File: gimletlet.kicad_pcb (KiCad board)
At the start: 4 copper layers, 58 x 57 mm, 59 parts, among them J1 Conn_02x16_Odd_Even, J2 Conn_02x15_Odd_Even, J3 Conn_01x04, J4 SWD, J5 I2C, SW1 RESET, U1 STM32H753IITx, Y1 8MHz

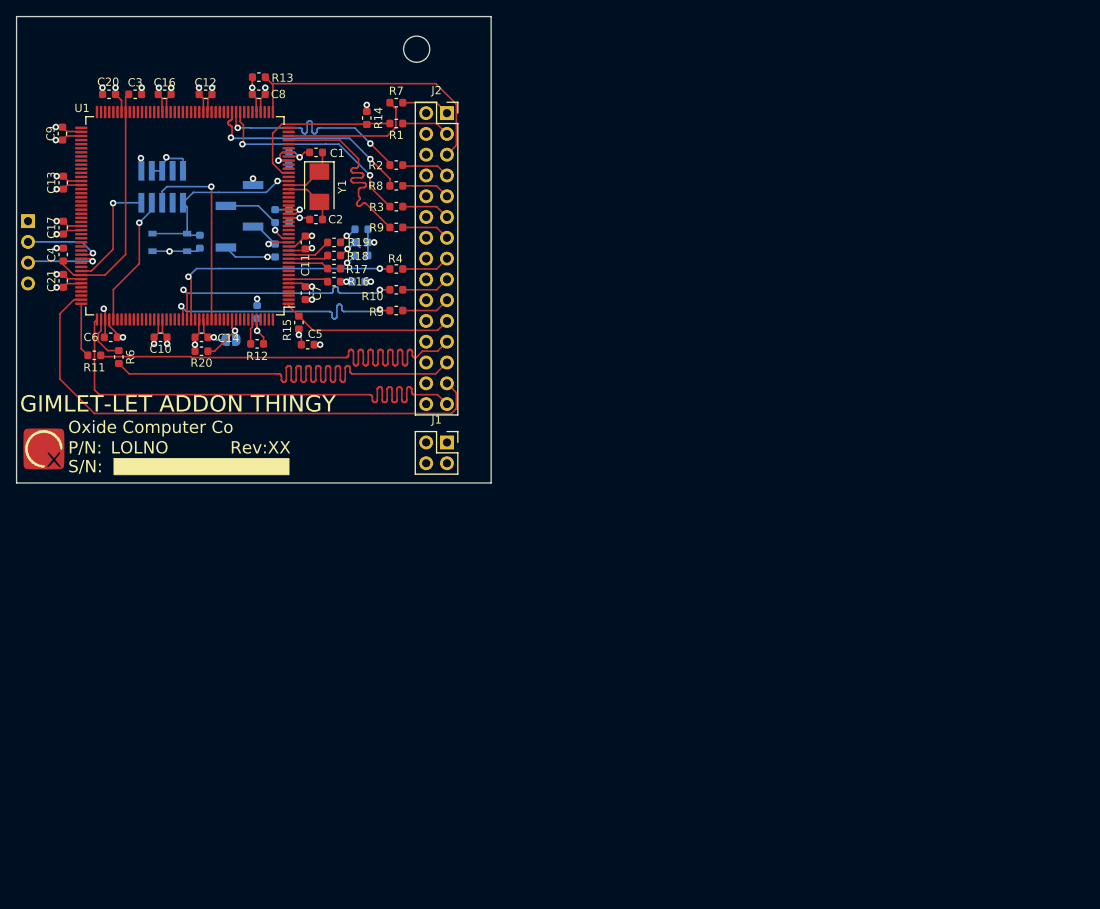
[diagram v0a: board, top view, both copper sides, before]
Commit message: gimletlet: revamp into useful board
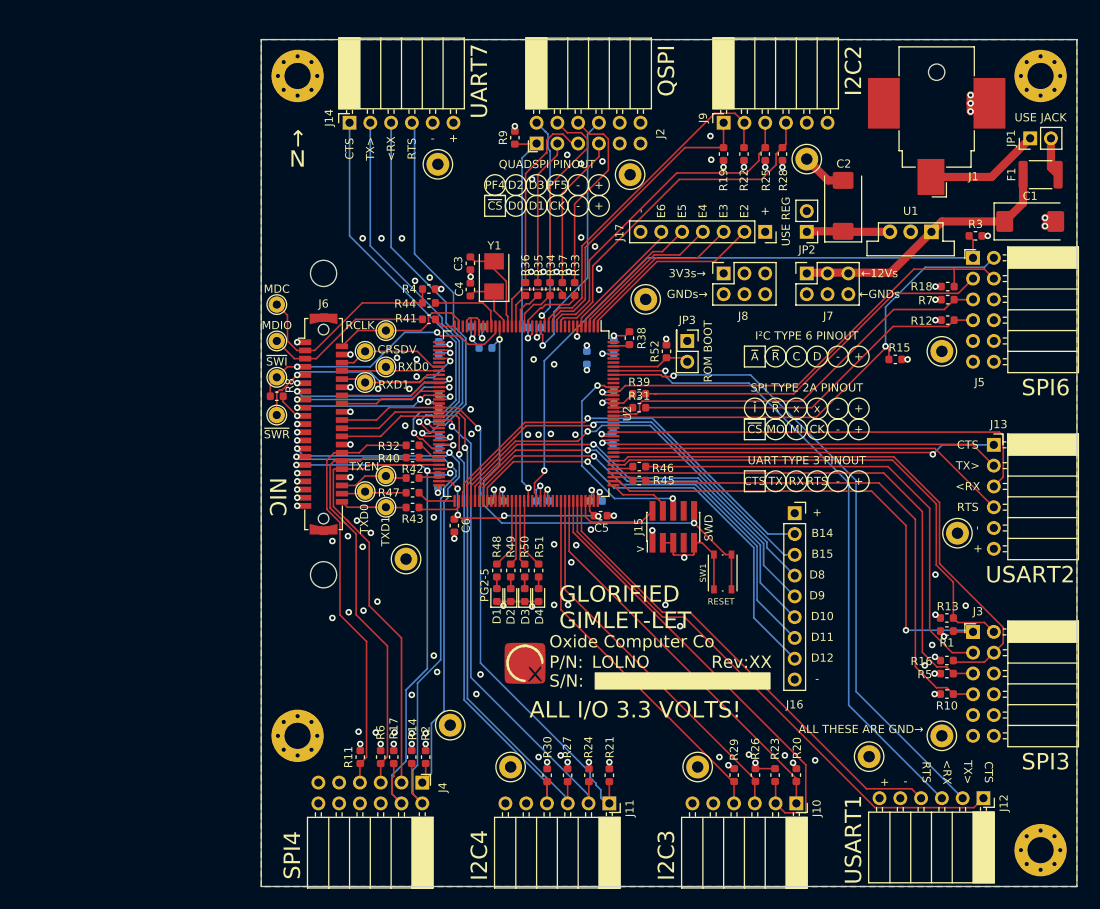
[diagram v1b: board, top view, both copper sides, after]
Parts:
- removed C21, C22: 0µ1, Capacitor_SMD:C_0603_1608Metric
- added F1: Polyfuse, Fuse:Fuse_1812_4532Metric, F.Cu at (184.2, 60.3)
- added H2: MountingHole, MountingHole:MountingHole_3.2mm_M3_Pad_Via, F.Cu at (184.2, 48.3)
- added H3: MountingHole, MountingHole:MountingHole_3.2mm_M3_Pad_Via, F.Cu at (184.2, 142.9)
- added H4: MountingHole, MountingHole:MountingHole_3.2mm_M3_Pad_Via, F.Cu at (93.3, 128.9)
- added H5: MountingHole, MountingHole:MountingHole_3.2mm_M3, F.Cu at (96.5, 72.4)
- added H6: MountingHole, MountingHole:MountingHole_3.2mm_M3, F.Cu at (96.5, 109.2)
- added J10: I2C3, pmod:PMOD_6pin_host_horizontal, F.Cu at (154.3, 137.2)
- added J11: I2C4, pmod:PMOD_6pin_host_horizontal, F.Cu at (131.4, 137.2)
- added J12: USART1, pmod:PMOD_6pin_host_horizontal, F.Cu at (177.2, 136.5)
- added J13: USART2, pmod:PMOD_6pin_host_horizontal, F.Cu at (178.4, 93.3)
- added J14: UART7, pmod:PMOD_6pin_host_horizontal, F.Cu at (99.7, 54.0)
- added J15: SWD, Connector_PinHeader_1.27mm:PinHeader_2x05_P1.27mm_Vertical_SMD, F.Cu at (139.3, 103.4)
- added J16: GPIO1, Connector_PinSocket_2.54mm:PinSocket_1x09_P2.54mm_Vertical, F.Cu at (154.1, 101.7)
- added J17: Conn_01x07, Connector_PinSocket_2.54mm:PinSocket_1x07_P2.54mm_Vertical, F.Cu at (150.5, 67.3)
- added J6: NIC, hirose-df9:Hirose_DF9-41S-1V(69)_2Rows_41Pin-2MP_P1.0mm_Vertical, F.Cu at (96.5, 90.8)
- added J7: 12V, Connector_PinSocket_2.54mm:PinSocket_2x03_P2.54mm_Vertical, F.Cu at (155.6, 72.4)
- added J8: 3V3, Connector_PinSocket_2.54mm:PinSocket_2x03_P2.54mm_Vertical, F.Cu at (145.4, 72.4)
- added J9: I2C2, pmod:PMOD_6pin_host_horizontal, F.Cu at (145.4, 54.0)
- added JP2: REG, Connector_PinHeader_2.54mm:PinHeader_1x02_P2.54mm_Vertical, F.Cu at (155.6, 67.3)
- added JP3: ROM, Connector_PinHeader_2.54mm:PinHeader_2x01_P2.54mm_Vertical, F.Cu at (141.0, 80.6)
- added R10: 10k, Resistor_SMD:R_0603_1608Metric, F.Cu at (172.7, 123.8)
- added R23: 10k, Resistor_SMD:R_0603_1608Metric, F.Cu at (151.7, 133.7)
- added R24: 10k, Resistor_SMD:R_0603_1608Metric, F.Cu at (128.9, 133.7)
- added R25: 10k, Resistor_SMD:R_0603_1608Metric, F.Cu at (150.5, 57.8)
- added R26: 10k, Resistor_SMD:R_0603_1608Metric, F.Cu at (149.3, 133.7)
- added R27: 10k, Resistor_SMD:R_0603_1608Metric, F.Cu at (126.3, 133.7)
- added R28: 10k, Resistor_SMD:R_0603_1608Metric, F.Cu at (152.6, 57.8)
- added R29: 10k, Resistor_SMD:R_0603_1608Metric, F.Cu at (146.7, 133.7)
- added R30: 10k, Resistor_SMD:R_0603_1608Metric, F.Cu at (123.8, 133.7)
- added R31: 22, Resistor_SMD:R_0603_1608Metric, F.Cu at (135.1, 88.8)
- added R32: 22, Resistor_SMD:R_0603_1608Metric, F.Cu at (107.4, 93.4)
- added R33: 22, Resistor_SMD:R_0603_1608Metric, F.Cu at (127.2, 74.3)
- added R34: 22, Resistor_SMD:R_0603_1608Metric, F.Cu at (124.2, 74.3)
- added R35: 22, Resistor_SMD:R_0603_1608Metric, F.Cu at (122.7, 74.3)
- added R36: 22, Resistor_SMD:R_0603_1608Metric, F.Cu at (121.2, 74.3)
- added R37: 22, Resistor_SMD:R_0603_1608Metric, F.Cu at (125.7, 74.3)
- added R38: 10k, Resistor_SMD:R_0603_1608Metric, F.Cu at (133.9, 80.3)
- added R39: 22, Resistor_SMD:R_0603_1608Metric, F.Cu at (135.1, 87.1)
- added R40: 22, Resistor_SMD:R_0603_1608Metric, F.Cu at (107.4, 94.9)
- added R41: 22, Resistor_SMD:R_0603_1608Metric, F.Cu at (109.4, 78.0)
- added R42: 22, Resistor_SMD:R_0603_1608Metric, F.Cu at (107.4, 97.4)
- added R44: 22, Resistor_SMD:R_0603_1608Metric, F.Cu at (109.4, 76.0)
- added R45: 22, Resistor_SMD:R_0603_1608Metric, F.Cu at (135.1, 97.7)
- added R46: 22, Resistor_SMD:R_0603_1608Metric, F.Cu at (135.1, 96.0)
- added R47: 22, Resistor_SMD:R_0603_1608Metric, F.Cu at (107.4, 99.2)
- added R48: 68, Resistor_SMD:R_0603_1608Metric, F.Cu at (117.7, 108.7)
- added R49: 68, Resistor_SMD:R_0603_1608Metric, F.Cu at (119.4, 108.7)
- added R50: 68, Resistor_SMD:R_0603_1608Metric, F.Cu at (121.1, 108.7)
- added R51: 68, Resistor_SMD:R_0603_1608Metric, F.Cu at (122.8, 108.7)
- added R52: 10k, Resistor_SMD:R_0603_1608Metric, F.Cu at (138.4, 81.9)
- added TP1: TestPoint_Small, TestPoint:TestPoint_THTPad_D2.0mm_Drill1.0mm, F.Cu at (90.8, 76.2)
- added TP10: TestPoint_Small, TestPoint:TestPoint_THTPad_D2.0mm_Drill1.0mm, F.Cu at (104.1, 83.8)
- added TP11: TestPoint_Small, TestPoint:TestPoint_THTPad_D2.0mm_Drill1.0mm, F.Cu at (101.6, 85.7)
- added TP12: GND, TestPoint:TestPoint_Loop_D3.50mm_Drill1.4mm_Beaded, F.Cu at (110.5, 59.1)
- added TP13: GND, TestPoint:TestPoint_Loop_D3.50mm_Drill1.4mm_Beaded, F.Cu at (134.0, 60.3)
- added TP14: GND, TestPoint:TestPoint_Loop_D3.50mm_Drill1.4mm_Beaded, F.Cu at (155.6, 58.4)
- added TP15: GND, TestPoint:TestPoint_Loop_D3.50mm_Drill1.4mm_Beaded, F.Cu at (172.1, 81.9)
- added TP16: GND, TestPoint:TestPoint_Loop_D3.50mm_Drill1.4mm_Beaded, F.Cu at (174.0, 104.1)
- added TP17: GND, TestPoint:TestPoint_Loop_D3.50mm_Drill1.4mm_Beaded, F.Cu at (172.1, 128.9)
- added TP18: GND, TestPoint:TestPoint_Loop_D3.50mm_Drill1.4mm_Beaded, F.Cu at (163.2, 131.4)
- added TP19: GND, TestPoint:TestPoint_Loop_D3.50mm_Drill1.4mm_Beaded, F.Cu at (142.2, 132.7)
- added TP2: TestPoint_Small, TestPoint:TestPoint_THTPad_D2.0mm_Drill1.0mm, F.Cu at (90.8, 80.6)
- added TP20: GND, TestPoint:TestPoint_Loop_D3.50mm_Drill1.4mm_Beaded, F.Cu at (119.4, 132.7)
- added TP21: GND, TestPoint:TestPoint_Loop_D3.50mm_Drill1.4mm_Beaded, F.Cu at (112.0, 127.6)
- added TP22: GND, TestPoint:TestPoint_Loop_D3.50mm_Drill1.4mm_Beaded, F.Cu at (106.6, 107.3)
- added TP23: GND, TestPoint:TestPoint_Loop_D3.50mm_Drill1.4mm_Beaded, F.Cu at (135.9, 75.6)
- added TP3: TestPoint_Small, TestPoint:TestPoint_THTPad_D2.0mm_Drill1.0mm, F.Cu at (90.8, 85.1)
- added TP4: TestPoint_Small, TestPoint:TestPoint_THTPad_D2.0mm_Drill1.0mm, F.Cu at (90.8, 89.7)
- added TP5: TestPoint_Small, TestPoint:TestPoint_THTPad_D2.0mm_Drill1.0mm, F.Cu at (104.1, 97.2)
- added TP6: TestPoint_Small, TestPoint:TestPoint_THTPad_D2.0mm_Drill1.0mm, F.Cu at (101.6, 99.1)
- added TP7: TestPoint_Small, TestPoint:TestPoint_THTPad_D2.0mm_Drill1.0mm, F.Cu at (104.1, 101.0)
- added TP8: TestPoint_Small, TestPoint:TestPoint_THTPad_D2.0mm_Drill1.0mm, F.Cu at (104.1, 79.4)
- added TP9: TestPoint_Small, TestPoint:TestPoint_THTPad_D2.0mm_Drill1.0mm, F.Cu at (101.6, 81.9)
- added U1: OKI-78SR-3.3_1.5-W36-C, Converter_DCDC:Converter_DCDC_muRata_OKI-78SR_Vertical, F.Cu at (170.8, 67.3)
- C1, C2: value 11p -> 22µ; footprint Capacitor_SMD:C_0603_1608Metric -> Capacitor_Tantalum_SMD:CP_EIA-7343-31_Kemet-D
- C10, C11, C12, C13, C14, C16, C17, C20, C8, C9: moved to B.Cu
- C3, C4: value 2µ2 100mR -> 11p
- C5: value 4µ7 -> 2µ2 100mR
- C6: value 0µ1 -> 2µ2 100mR
- C7: value 0µ1 -> 4µ7; moved to B.Cu
- D1, D2, D3, D4, R21, R22, SW1: moved to F.Cu
- H1: footprint MountingHole:MountingHole_3.2mm_M3 -> MountingHole:MountingHole_3.2mm_M3_Pad_Via; moved to F.Cu
- J1: value Conn_02x16_Odd_Even -> 12V; footprint Connector_PinSocket_2.54mm:PinSocket_2x02_P2.54mm_Vertical -> Connector_BarrelJack:BarrelJack_CUI_PJ-036AH-SMT_Horizontal
- J2: value Conn_02x15_Odd_Even -> QSPI; footprint Connector_PinSocket_2.54mm:PinSocket_2x15_P2.54mm_Vertical -> pmod:PMOD_12pin_host_horizontal
- J3: value Conn_01x04 -> SPI3; footprint Connector_PinHeader_2.54mm:PinHeader_1x04_P2.54mm_Horizontal -> pmod:PMOD_12pin_host_horizontal; moved to F.Cu
- J4: value SWD -> SPI4; footprint Connector_PinHeader_1.27mm:PinHeader_2x05_P1.27mm_Vertical_SMD -> pmod:PMOD_12pin_host_horizontal; moved to F.Cu
- J5: value I2C -> SPI6; footprint Connector_PinHeader_2.54mm:PinHeader_1x04_P2.54mm_Vertical_SMD_Pin1Left -> pmod:PMOD_12pin_host_horizontal; moved to F.Cu
- JP1: value ROM -> JACK; footprint Jumper:SolderJumper-2_P1.3mm_Open_RoundedPad1.0x1.5mm -> Connector_PinHeader_2.54mm:PinHeader_1x02_P2.54mm_Vertical; moved to F.Cu
- R1, R11, R2, R3, R5, R6, R7, R9: value 22 -> 10k
- R13, R14, R15: value 100k -> 10k
- R16, R17, R18, R19: value 68 -> 10k
- R4, R8: value 22 -> 100k
- U2: renamed from U1; value STM32H753IITx -> STM32H753ZITx; footprint Package_QFP:LQFP-176_24x24mm_P0.5mm -> Package_QFP:LQFP-144_20x20mm_P0.5mm
- moved J3 125.9 mm to (175.9, 116.2), turned to 0 degrees
- moved R13 107.0 mm to (172.7, 114.5), turned to 180 degrees
- moved JP1 100.7 mm to (182.9, 55.9), turned to 90 degrees
- moved R1 91.5 mm to (172.7, 116.1), turned to 180 degrees
- moved J5 89.8 mm to (175.9, 70.5)
- moved R20 89.3 mm to (154.3, 133.7), turned to 90 degrees
- moved R16 88.1 mm to (172.7, 119.7)
- moved C1 87.7 mm to (182.9, 66.0), turned to 0 degrees
- moved R12 84.4 mm to (172.8, 78.1), turned to 180 degrees
- moved R5 80.6 mm to (172.7, 121.3), turned to 180 degrees
- moved J4 79.5 mm to (108.6, 134.6)
- moved SW1 78.8 mm to (145.3, 109.0), turned to 270 degrees
- moved R14 78.3 mm to (107.3, 131.5), turned to 90 degrees
- moved R21 76.0 mm to (131.4, 133.7), turned to 90 degrees
- moved R18 75.1 mm to (172.8, 74.0)
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- renumbered R10 to R43
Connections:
- C1 pad 1: /OSC_OUT -> +12V
- C2 pad 1: /OSC_IN -> /REG_3V3
- C20 pad 1: +3V3 -> /~RST
- C3 pad 1: Net-(C3-Pad1) -> /OSC_IN
- C4 pad 1: Net-(C3-Pad1) -> /OSC_OUT
- C5 pad 1: +3V3 -> Net-(C5-Pad1)
- C6 pad 1: +3V3 -> Net-(C5-Pad1)
- H1 pad 1: (no net) -> GND
- J1 pad 1: +3V3 -> /JACK_12V
- J1 pad 2: Net-(J1-Pad2) -> GND
- J1 pad 3: +3V3 -> Net-(J1-Pad3)
- J2 pad 1: /X_MDIO -> /~QSPI_CS
- J2 pad 10: GND -> /QSPI_XTRA10
- J2 pad 11: /X_RMII_CRS_DV -> GND
- J2 pad 12: GND -> +3V3
- J2 pad 2: GND -> /QSPI_IO0
- J2 pad 3: /X_MDC -> /QSPI_IO1
- J2 pad 4: GND -> /QSPI_CLK
- J2 pad 5: /~SMI_IRQ -> GND
- J2 pad 6: GND -> +3V3
- J2 pad 7: /X_RMII_RXD0 -> /QSPI_XTRA7
- J2 pad 8: GND -> /QSPI_IO2
- J2 pad 9: /X_RMII_RXD1 -> /QSPI_IO3
- J3 pad 1: +3V3 -> /~SPI3_CS
- J3 pad 2: /USART1_TX -> /SPI3_MOSI
- J3 pad 3: /USART1_RX -> /SPI3_MISO
- J3 pad 4: GND -> /SPI3_SCK
- J4 pad 1: +3V3 -> /~SPI4_CS
- J4 pad 10: /~RST -> Net-(J4-Pad10)
- J4 pad 2: /SWDIO -> /SPI4_MOSI
- J4 pad 3: GND -> /SPI4_MISO
- J4 pad 4: /SWCLK -> /SPI4_SCK
- J4 pad 6: /SWO -> +3V3
- J4 pad 7: Net-(J4-Pad7) -> /~SPI4_INT
- J4 pad 8: Net-(J4-Pad8) -> /~SPI4_RESET
- J4 pad 9: GND -> Net-(J4-Pad9)
- J5 pad 1: +3V3 -> /~SPI6_CS
- J5 pad 2: /SDA -> /SPI6_MOSI
- J5 pad 3: /SCL -> /SPI6_MISO
- J5 pad 4: GND -> /SPI6_SCK
- JP1 pad 1: +3V3 -> /JACK_12V
- JP1 pad 2: /BOOT0 -> /12V_IN
- R1 pad 1: /MDC -> /~SPI3_CS
- R1 pad 2: /X_MDC -> +3V3
- R11 pad 1: /SPI2_SCK -> /SPI4_SCK
- R11 pad 2: /X_SPI_SCK -> +3V3
- R12 pad 1: Net-(R12-Pad1) -> /SPI6_SCK
- R13 pad 1: +3V3 -> /~SPI3_INT
- R13 pad 2: /~SMI_IRQ -> +3V3
- R14 pad 1: +3V3 -> /~SPI4_INT
- R14 pad 2: /MDC -> +3V3
- R15 pad 1: +3V3 -> /~SPI6_INT
- R15 pad 2: /~SW_IRQ -> +3V3
- R16 pad 1: Net-(D1-Pad2) -> /~SPI3_RESET
- R16 pad 2: /LED0 -> +3V3
- R17 pad 1: Net-(D2-Pad2) -> /~SPI4_RESET
- R17 pad 2: /LED1 -> +3V3
- R18 pad 1: Net-(D3-Pad2) -> /~SPI6_RESET
- R18 pad 2: /LED2 -> +3V3
- R19 pad 1: Net-(D4-Pad2) -> /~I2C2_SMBA
- R19 pad 2: /LED3 -> +3V3
- R2 pad 1: /RMII_RXD0 -> /~SPI4_CS
- R2 pad 2: /X_RMII_RXD0 -> +3V3
- R20 pad 1: /BOOT0 -> /~I2C3_SMBA
- R20 pad 2: GND -> +3V3
- R21 pad 1: /SDA -> /~I2C4_SMBA
- R22 pad 1: /SCL -> /~I2C2_RESET
- R3 pad 1: /RMII_CRS_DV -> /~SPI6_CS
- R3 pad 2: /X_RMII_CRS_DV -> +3V3
- R4 pad 1: /RMII_TXD0 -> +3V3
- R4 pad 2: /X_RMII_TXD0 -> /MDC
- R43 pad 2: /X_RMII_TXD1 -> Net-(R43-Pad2)
- R5 pad 1: /RMII_TXEN -> /SPI3_MISO
- R5 pad 2: /X_RMII_TXEN -> +3V3
- R6 pad 1: /SPI2_MOSI -> /SPI4_MISO
- R6 pad 2: /X_SPI_MOSI -> +3V3
- R7 pad 1: /MDIO -> /SPI6_MISO
- R7 pad 2: /X_MDIO -> +3V3
- R8 pad 1: /RMII_RXD1 -> +3V3
- R8 pad 2: /X_RMII_RXD1 -> /~SMI_IRQ
- R9 pad 1: /RMII_REF_CLK -> /~QSPI_CS
- R9 pad 2: /X_RMII_REFCLK -> +3V3
- U2 pad 1: /~SW_IRQ -> /PE2
- U2 pad 10: Net-(U1-Pad10) -> /I2C2_SDA
- U2 pad 100: Net-(U1-Pad100) -> /I2C3_SCL
- U2 pad 101: Net-(U1-Pad101) -> /~I2C3_SMBA
- U2 pad 102: GND -> /~I2C3_RESET
- U2 pad 103: +3V3 -> /USART1_CTS
- U2 pad 104: Net-(U1-Pad104) -> /USART1_RTS
- U2 pad 105: Net-(U1-Pad105) -> /SWDIO
- U2 pad 106: Net-(U1-Pad106) -> Net-(C5-Pad1)
- U2 pad 107: Net-(U1-Pad107) -> GND
- U2 pad 108: Net-(U1-Pad108) -> +3V3
- U2 pad 109: Net-(U1-Pad109) -> /SWCLK
- U2 pad 11: /LED1 -> /I2C2_SCL
- U2 pad 110: Net-(U1-Pad110) -> /~SPI3_CS
- U2 pad 112: Net-(U1-Pad112) -> /SPI3_MISO
- U2 pad 113: GND -> Net-(R46-Pad2)
- U2 pad 114: +3V3 -> /~SPI3_INT
- U2 pad 115: Net-(U1-Pad115) -> /~SPI3_RESET
- U2 pad 117: Net-(U1-Pad117) -> /USART2_CTS
- U2 pad 118: Net-(U1-Pad118) -> /USART2_RTS
- U2 pad 119: Net-(U1-Pad119) -> /USART2_TX
- U2 pad 12: /LED2 -> /~I2C2_SMBA
- U2 pad 120: /USART1_TX -> GND
- U2 pad 121: /USART1_RX -> +3V3
- U2 pad 122: Net-(U1-Pad122) -> /USART2_RX
- U2 pad 124: /SWDIO -> Net-(U2-Pad124)
- U2 pad 125: Net-(C3-Pad1) -> Net-(U2-Pad125)
- U2 pad 126: GND -> /~SPI6_INT
- U2 pad 127: +3V3 -> /SPI6_MISO
- U2 pad 13: /LED3 -> /~I2C2_RESET
- U2 pad 130: Net-(U1-Pad130) -> GND
- U2 pad 131: /~SPI2_CS0 -> +3V3
- U2 pad 132: /SPI2_SCK -> /~SPI6_RESET
- U2 pad 133: /SPI2_MISO -> /SWO
- U2 pad 134: /SPI2_MOSI -> Net-(U2-Pad134)
- U2 pad 135: GND -> Net-(U2-Pad135)
- U2 pad 136: +3V3 -> /USART1_TX
- U2 pad 137: /SWCLK -> /USART1_RX
- U2 pad 138: Net-(U1-Pad138) -> /BOOT0
- U2 pad 14: GND -> /QSPI_XTRA7
- U2 pad 144: Net-(U1-Pad144) -> +3V3
- U2 pad 15: +3V3 -> /QSPI_XTRA10
- U2 pad 16: /SDA -> GND
- U2 pad 17: /SCL -> +3V3
- U2 pad 2: Net-(U1-Pad2) -> /PE3
- U2 pad 22: GND -> Net-(R37-Pad1)
- U2 pad 23: +3V3 -> /OSC_IN
- U2 pad 24: Net-(U1-Pad24) -> /OSC_OUT
- U2 pad 25: Net-(U1-Pad25) -> /~RST
- U2 pad 26: Net-(U1-Pad26) -> /~SMI_IRQ
- U2 pad 29: /OSC_IN -> Net-(U2-Pad29)
- U2 pad 3: Net-(U1-Pad3) -> /PE4
- U2 pad 30: /OSC_OUT -> +3V3
- U2 pad 31: /~RST -> GND
- U2 pad 32: Net-(U1-Pad32) -> +3V3
- U2 pad 33: /MDC -> +3V3
- U2 pad 35: Net-(U1-Pad35) -> /RMII_REF_CLK
- U2 pad 36: +3V3 -> Net-(R41-Pad1)
- U2 pad 37: GND -> Net-(U2-Pad37)
- U2 pad 38: +3V3 -> GND
- U2 pad 4: Net-(U1-Pad4) -> /PE5
- U2 pad 41: /RMII_REF_CLK -> /~SMI_RESET
- U2 pad 42: /MDIO -> Net-(U2-Pad42)
- U2 pad 43: Net-(U1-Pad43) -> /RMII_CRS_DV
- U2 pad 44: Net-(U1-Pad44) -> /RMII_RXD0
- U2 pad 45: /~SMI_IRQ -> /RMII_RXD1
- U2 pad 46: Net-(U1-Pad46) -> /PB0
- U2 pad 47: Net-(U1-Pad47) -> /PB1
- U2 pad 48: GND -> /PB2
- U2 pad 49: +3V3 -> /PF11
- U2 pad 5: Net-(U1-Pad5) -> /PE6
- U2 pad 50: Net-(U1-Pad50) -> /PF12
- U2 pad 51: Net-(U1-Pad51) -> GND
- U2 pad 52: Net-(U1-Pad52) -> +3V3
- U2 pad 53: /RMII_CRS_DV -> /~I2C4_SMBA
- U2 pad 54: /RMII_RXD0 -> /I2C4_SCL
- U2 pad 55: /RMII_RXD1 -> /I2C4_SDA
- U2 pad 56: Net-(U1-Pad56) -> /~I2C4_RESET
- U2 pad 58: Net-(U1-Pad58) -> /UART7_RX
- U2 pad 59: Net-(U1-Pad59) -> /UART7_TX
- U2 pad 60: Net-(U1-Pad60) -> /UART7_RTS
- U2 pad 63: Net-(U1-Pad63) -> /UART7_CTS
- U2 pad 64: Net-(U1-Pad64) -> /~SPI4_CS
- U2 pad 67: Net-(U1-Pad67) -> /SPI4_MOSI
- U2 pad 68: Net-(U1-Pad68) -> /~SPI4_INT
- U2 pad 69: Net-(U1-Pad69) -> /~SPI4_RESET
- U2 pad 7: /LED0 -> Net-(U2-Pad7)
- U2 pad 71: GND -> Net-(C5-Pad1)
- U2 pad 74: Net-(U1-Pad74) -> Net-(R43-Pad2)
- U2 pad 75: Net-(U1-Pad75) -> /PB14
- U2 pad 76: Net-(U1-Pad76) -> /PB15
- U2 pad 77: Net-(U1-Pad77) -> /PD8
- U2 pad 78: Net-(U1-Pad78) -> /PD9
- U2 pad 79: Net-(U1-Pad79) -> /PD10
- U2 pad 80: Net-(U1-Pad80) -> /PD11
- U2 pad 81: Net-(C3-Pad1) -> /PD12
- U2 pad 82: +3V3 -> Net-(U2-Pad82)
- U2 pad 83: Net-(U1-Pad83) -> GND
- U2 pad 84: Net-(U1-Pad84) -> +3V3
- U2 pad 87: Net-(U1-Pad87) -> /LED0
- U2 pad 88: Net-(U1-Pad88) -> /LED1
- U2 pad 89: Net-(U1-Pad89) -> /LED2
- U2 pad 90: GND -> /LED3
- U2 pad 91: +3V3 -> /~QSPI_CS
- U2 pad 93: Net-(U1-Pad93) -> /~SPI6_CS
- U2 pad 94: Net-(U1-Pad94) -> GND
- U2 pad 95: Net-(U1-Pad95) -> +3V3
- U2 pad 99: Net-(U1-Pad99) -> /I2C3_SDA
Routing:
- net /~SPI6_CS: track 0.00 -> 78.2 mm, vias 0 -> 1
- net /~I2C4_SMBA: track 0.00 -> 74.0 mm, vias 0 -> 1
- net /~SPI4_INT: track 0.00 -> 71.6 mm, vias 0 -> 2
- net /I2C4_SCL: track 0.00 -> 71.1 mm, vias 0 -> 1
- net /~SPI3_RESET: track 0.00 -> 69.9 mm
- net /I2C4_SDA: track 0.00 -> 69.7 mm, vias 0 -> 1
- net /USART1_TX: track 10.0 -> 79.4 mm
- net /USART1_RX: track 9.49 -> 78.1 mm
- net /USART1_CTS: track 0.00 -> 67.8 mm
- net /~SPI4_RESET: track 0.00 -> 67.3 mm, vias 0 -> 2
- net /~SPI4_CS: track 0.00 -> 66.9 mm, vias 0 -> 2
- net /X_SPI_SCK: track 65.3 -> 0.00 mm
- net /SPI2_MISO: track 65.3 -> 0.00 mm
- net /~SPI2_CS0: track 65.3 -> 0.00 mm
- net /X_SPI_MOSI: track 65.3 -> 0.00 mm
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- added copper zone on In2.Cu, net +3V3
- added copper zone on B.Cu, net GND
- added copper zone on F.Cu, net GND
- added copper zone on In1.Cu, net GND
- removed copper zone on In1.Cu, net +3V3
- removed copper zone on In2.Cu, net GND
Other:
- board size 58 x 57 mm -> 99.7 x 103.5 mm
- board text added: "3V3s→"
- board text added: ">"
- board text added: "ALL I/O 3.3 VOLTS!"
- board text added: "ALL THESE ARE GND→"
- board text added: "B14"
- board text added: "B15"
- board text added: "CK"
- board text added: "CRSDV"
- board text added: "CTS"
- board text added: "D0"
- board text added: "D1"
- board text added: "D10"
- board text added: "D11"
- board text added: "D12"
- board text added: "D2"
- board text added: "D3"
- board text added: "D8"
- board text added: "D9"
- board text added: "E2"
- board text added: "E3"
- board text added: "E4"
- board text added: "E5"
- board text added: "E6"
- board text added: "GLORIFIED GIMLET-LET"
- board text added: "GNDs→"
- board text added: "I2C2"
- board text added: "I2C3"
- board text added: "I2C4"
- board text added: "I²C TYPE 6 PINOUT"
- board text added: "MI"
- board text added: "MO"
- board text added: "N"
- board text added: "NIC"
- board text added: "PF4"
- board text added: "PF5"
- board text added: "PG2-5"
- board text added: "QSPI"
- board text added: "QUADSPI PINOUT"
- board text added: "ROM BOOT"
- board text added: "RTS"
- board text added: "RX"
- board text added: "SPI TYPE 2A PINOUT"
- board text added: "SPI3"
- board text added: "SPI4"
- board text added: "SPI6"
- board text added: "TX"
- board text added: "UART TYPE 3 PINOUT"
- board text added: "UART7"
- board text added: "USART1"
- board text added: "USART2"
- board text added: "USE JACK"
- board text added: "USE REG"
- board text added: "x"
- board text added: "~A"
- board text added: "~I"
- board text added: "~R"
- board text added: "~SWI"
- board text added: "~SWR"
- board text added: "←12Vs"
- board text added: "←GNDs"
- board text added: "→"
- board text removed: "+3"
- board text removed: "+3.3"
- board text removed: "DV"
- board text removed: "GIMLET-LET ADDON THINGY"
- board text removed: "GND"
- board text removed: "I2C YAY"
- board text removed: "LEDS: PI8-11"
- board text removed: "MISO"
- board text removed: "MOSI"
- board text removed: "RX=PA10"
- board text removed: "SCK"
- board text removed: "TX=PA9"
- board text removed: "~SMIQ"
- board text removed: "~SWQ"
- board text removed: "← SHORT THIS AT RESET FOR BOOTLOADER"
- board text removed: "←THIS HOLE SHOULD LINE UP WITH A MATCHING ONE"
- board text removed: "←USART1"
- board text removed: "↑SPI TO SWITCH"
- board text removed: "↓RMII"
